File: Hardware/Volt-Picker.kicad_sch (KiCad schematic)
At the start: 60 parts, among them J1 USB_C_Receptacle, J2 Conn_01x02_Pin, Q1 SQS840CENW, Q2 MMBT2222A, Q5 SQS840CENW, U1 AP33771CFBZ-13-FA01

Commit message: ...
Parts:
- D1, D2, D3, D4: footprint tinker:PGB1010603NRHF -> LCSCfootprints:PGB1010603NRHF
- J1: footprint tinker:USB_C_Receptacle_HRO_TYPE-C-31-M-12 -> TINKERfootprints:USB_C_Receptacle_HRO_TYPE-C-31-M-12
- J2: footprint tinker:TerminalBlock_DG350-3.5-02P-14-00A(H) -> TINKERfootprints:TerminalBlock_DG350-3.5-02P-14-00A(H)
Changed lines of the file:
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@@
 			)
 		)
-		(property "Footprint" "tinker:PGB1010603NRHF"
+		(property "Footprint" "LCSCfootprints:PGB1010603NRHF"
 			(at 66.04 39.37 0)
 			(effects
@@
 			)
 		)
-		(property "Footprint" "tinker:PGB1010603NRHF"
+		(property "Footprint" "LCSCfootprints:PGB1010603NRHF"
 			(at 66.04 69.85 0)
 			(effects
@@
 			)
 		)
-		(property "Footprint" "tinker:TerminalBlock_DG350-3.5-02P-14-00A(H)"
+		(property "Footprint" "TINKERfootprints:TerminalBlock_DG350-3.5-02P-14-00A(H)"
 			(at 250.19 25.4 0)
 			(effects
@@
 			)
 		)
-		(property "Footprint" "tinker:PGB1010603NRHF"
+		(property "Footprint" "LCSCfootprints:PGB1010603NRHF"
 			(at 66.04 49.53 0)
 			(effects
@@
 			)
 		)
-		(property "Footprint" "tinker:PGB1010603NRHF"
+		(property "Footprint" "LCSCfootprints:PGB1010603NRHF"
 			(at 66.04 59.69 0)
 			(effects
@@
 			)
 		)
-		(property "Footprint" "tinker:USB_C_Receptacle_HRO_TYPE-C-31-M-12"
+		(property "Footprint" "TINKERfootprints:USB_C_Receptacle_HRO_TYPE-C-31-M-12"
 			(at 33.02 50.8 0)
 			(effects

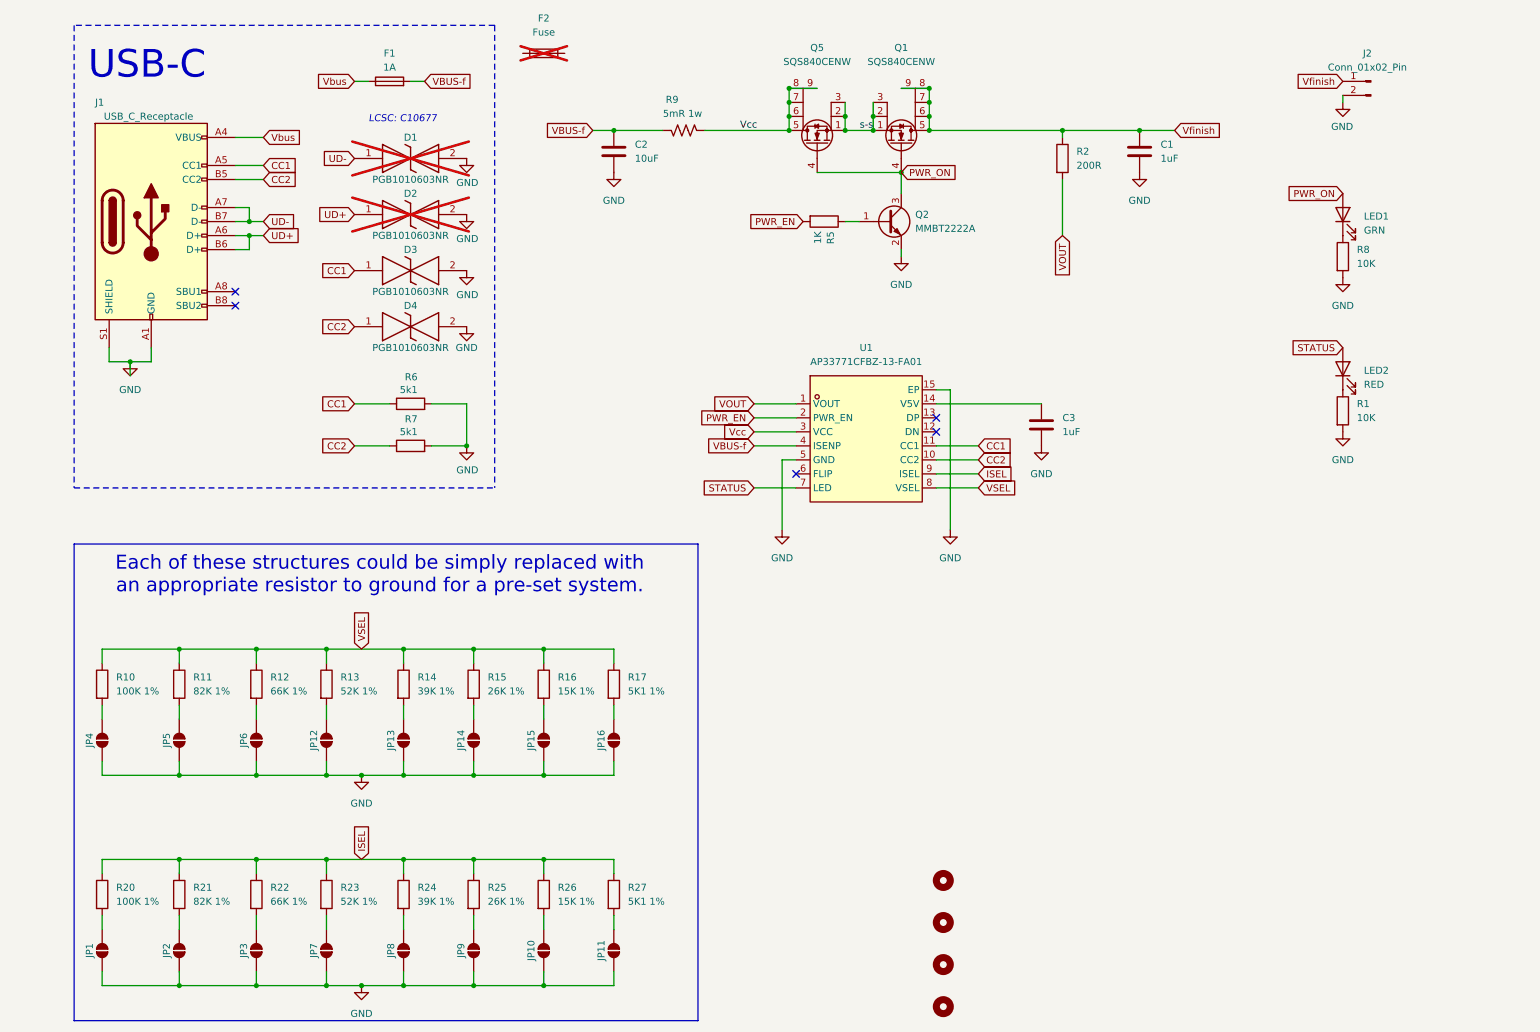
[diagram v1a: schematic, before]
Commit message: Tweakin' & Squishin'
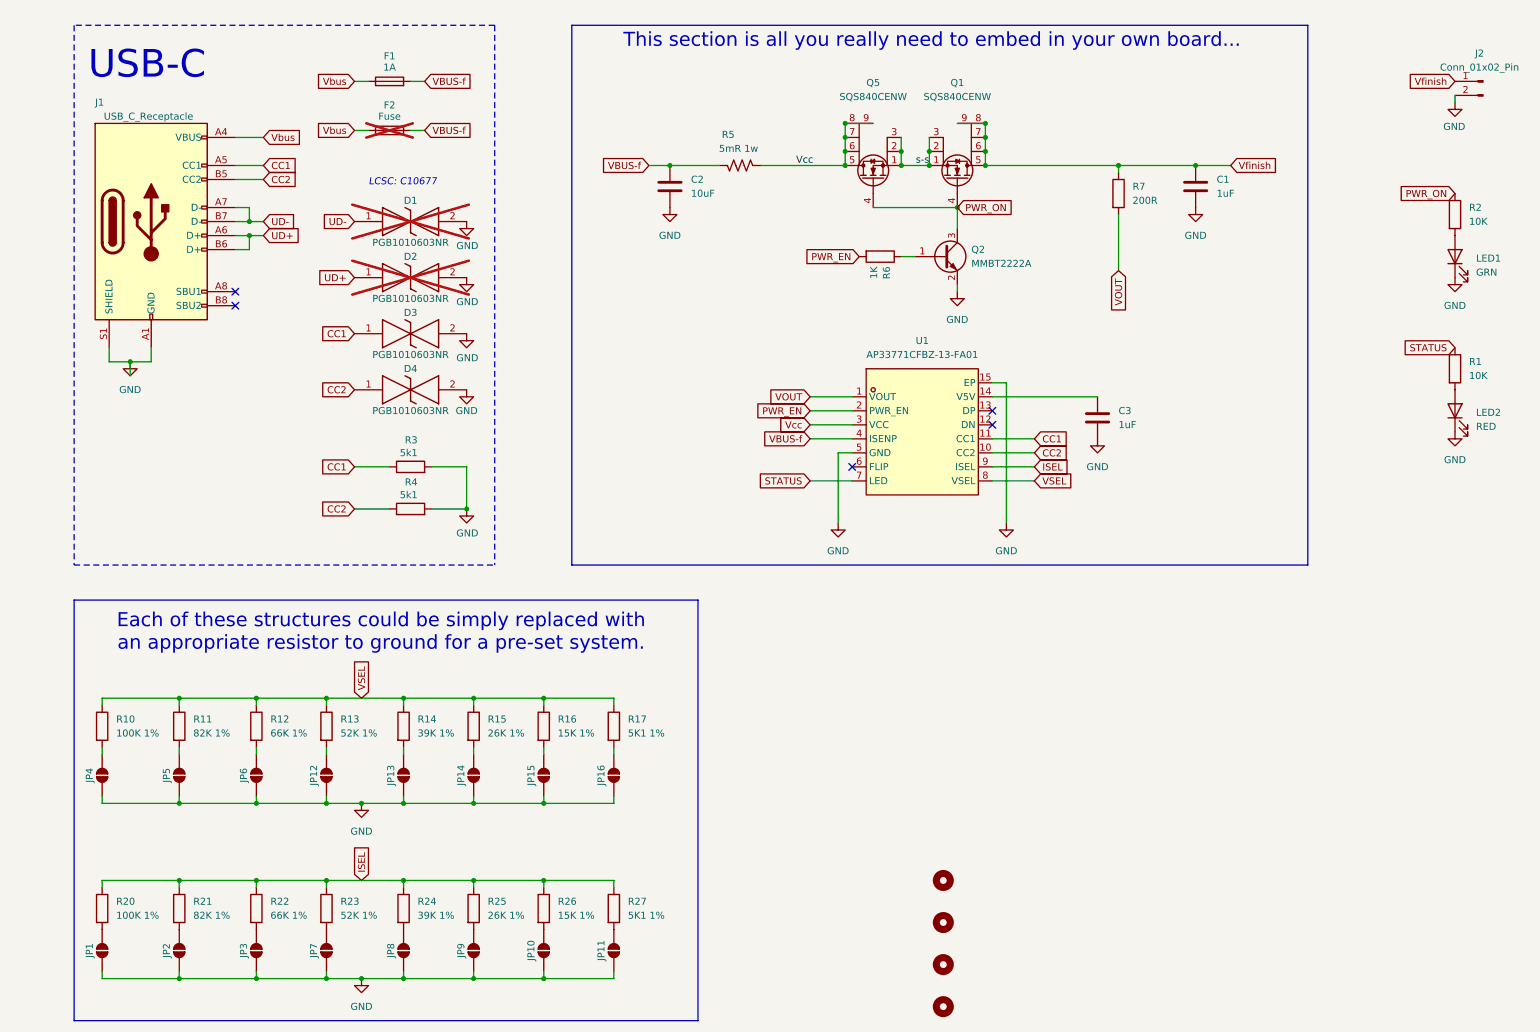
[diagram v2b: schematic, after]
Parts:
- renumbered R8 to R2, R6 to R3, R7 to R4, R9 to R5, R5 to R6, R2 to R7
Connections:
- net GND: now also LED1.1 (K), LED2.1 (K); no longer R1.2, R2.2
- net PWR_ON: now also R2.1; no longer LED1.2 (A)
- net STATUS: now also R1.1; no longer LED2.2 (A)
- net VBUS-f: now also F2.1
- net Vbus: now also F2.2
- new net: LED1.2 (A), R2.2
- new net: LED2.2 (A), R1.2
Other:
- note added: "This section is all you really need to embed in your own board..."
- moved on the sheet: C1, C2, C3, D1, D2, D3, D4, F2, J2, JP12, JP13, JP14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
